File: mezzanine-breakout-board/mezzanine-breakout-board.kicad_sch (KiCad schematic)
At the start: 2 parts, among them J1 Mezzanine Plug, J2 Conn_01x10

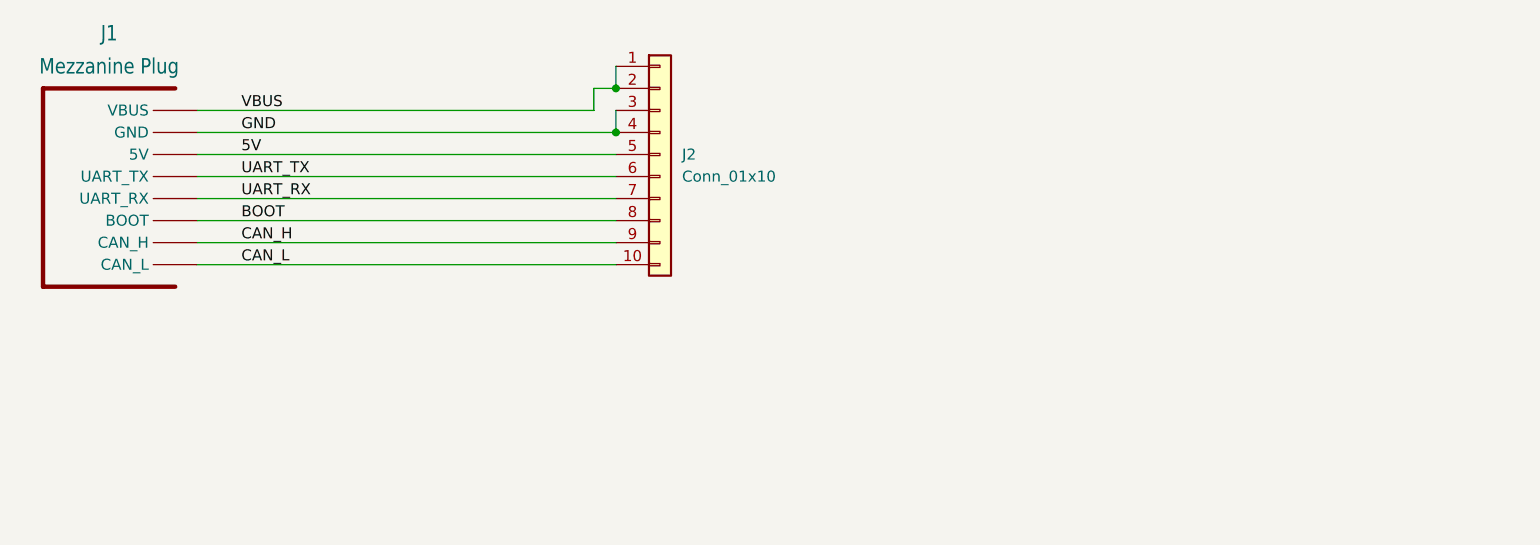
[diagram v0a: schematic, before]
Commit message: version, date, and possibly other changes and switched to v8
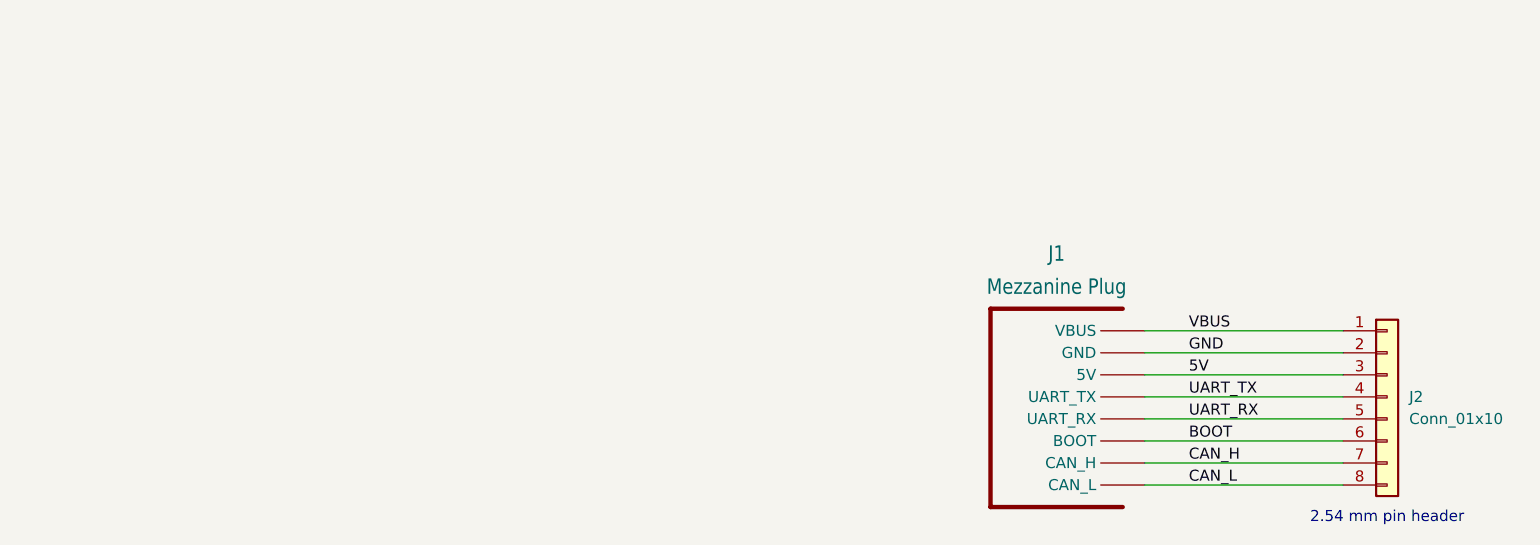
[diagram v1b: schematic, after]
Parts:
- J2: footprint Connector_PinHeader_2.54mm:PinHeader_1x10_P2.54mm_Vertical -> Connector_PinHeader_2.54mm:PinHeader_1x08_P2.54mm_Vertical; symbol Connector_Generic:Conn_01x10 -> Connector_Generic:Conn_01x08
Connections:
- net 5V: now also J2.3 (Pin_3); no longer J2.5 (Pin_5)
- net BOOT: now also J2.6 (Pin_6); no longer J2.8 (Pin_8)
- net CAN_H: now also J2.7 (Pin_7); no longer J2.9 (Pin_9)
- net CAN_L: now also J2.8 (Pin_8); no longer J2.10 (Pin_10)
- net GND: now also J2.2 (Pin_2); no longer J2.3 (Pin_3), J2.4 (Pin_4)
- net UART_RX: now also J2.5 (Pin_5); no longer J2.7 (Pin_7)
- net UART_TX: now also J2.4 (Pin_4); no longer J2.6 (Pin_6)
- net VBUS: no longer J2.2 (Pin_2)
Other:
- note added: "2.54 mm pin header"
- title: (none) -> OreSat Reaction Wheel Mezzanine Breakout
- moved on the sheet: J1
